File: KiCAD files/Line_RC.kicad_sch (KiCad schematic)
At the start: 67 parts, among them IC1 ESP32-WROVER-E-N4R8, IC2 CP2102N-A02-GQFN28R, IC3 BC847BDW1T1G, IC4 TLV75533PDBVR, IC5 TPS563240DDCR, J1 XT60PW-M, J2 XT60PW-M, J3 Conn_01x03_ESC, J4 FFC3B07-08-T, J6 Motor OUT, J7 Motor OUT, U3 DRV8213RTER, U4 DRV8213RTER

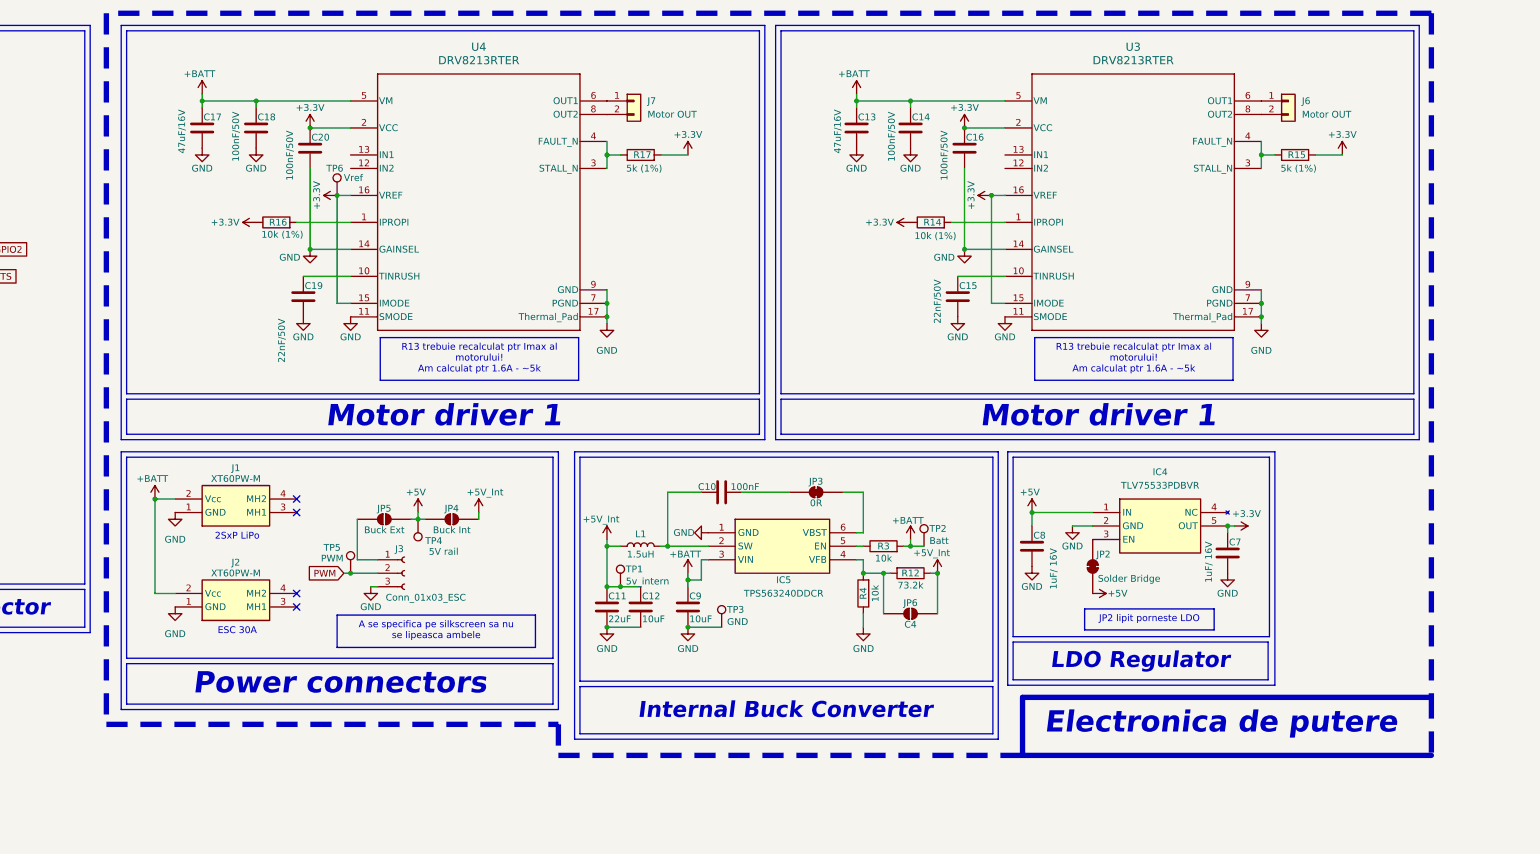
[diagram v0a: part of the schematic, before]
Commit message: added new motor driver
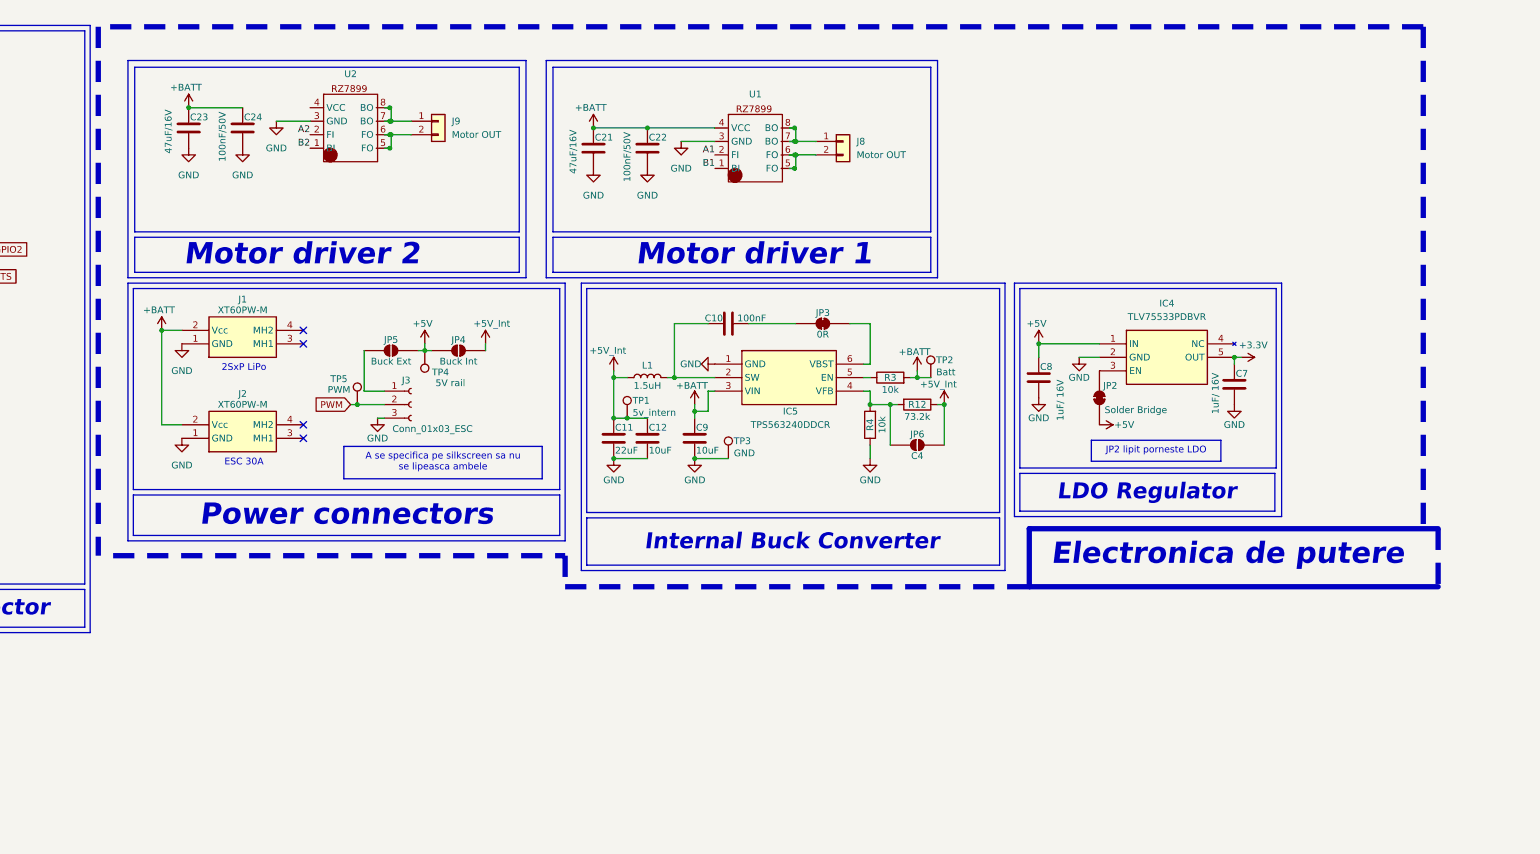
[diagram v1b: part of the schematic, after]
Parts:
- removed C13, C17: 47uF/16V, symbol Device:C
- removed C14, C16, C18, C20: 100nF/50V, symbol Device:C
- removed C15, C19: 22nF/50V, symbol Device:C
- removed J6, J7: Motor OUT, symbol Connector_Generic:Conn_01x02
- removed R14, R16: 10k (1%), symbol Device:R
- removed R15, R17: 5k (1%), symbol Device:R
- removed TP6: Vref, symbol Connector:TestPoint
- removed U3, U4: DRV8213RTER, RTE0016C-IPC_A, symbol 2026-07-26_14-19-18:DRV8213RTER
- added C21, C23: 47uF/16V, symbol Device:C
- added C22, C24: 100nF/50V, symbol Device:C
- added J8, J9: Motor OUT, symbol Connector_Generic:Conn_01x02
- added U1, U2: (no value), symbol RZ7899:RZ7899
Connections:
- net +BATT: now also C21.1, C22.1, C23.1, C24.1, U1.4 (VCC)
- net GND: now also C21.2, C22.2, C23.2, C24.2, U1.3 (GND), U2.3 (GND)
- new net: J9.1 (Pin_1), U2.7 (BO), U2.8 (BO)
- new net: J9.2 (Pin_2), U2.5 (FO), U2.6 (FO)
- new net: J8.1 (Pin_1), U1.7 (BO), U1.8 (BO)
- new net: J8.2 (Pin_2), U1.5 (FO), U1.6 (FO)
- new net A1: U1.2 (FI)
- new net A2: U2.2 (FI)
- new net B1: U1.1 (BI)
- new net B2: U2.1 (BI)
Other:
- note added: "Motor driver 2"
- moved on the sheet: C10, C11, C12, C7, C8, C9, IC4, IC5, J1, J2, J3, JP2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
